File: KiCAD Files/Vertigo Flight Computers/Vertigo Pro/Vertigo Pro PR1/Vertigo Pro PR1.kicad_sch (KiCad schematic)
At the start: 152 parts, among them IC1 ICM-20602, IC2 DPS310XTSA1, J1 ST-LINK Conn, J2 USB_C_Receptacle_USB2.0, J3 FFC2A32-24-T, J4 Screw_Terminal, J5 Screw_Terminal, J6 Screw_Terminal, J7 Screw_Terminal, Q1 IRF530SPBF, Q2 MMBT3904-TP, Q3 MMBT3904-TP, Q4 IRF530SPBF, Q5 SI7149ADP-T1-GE3, Q6 MMBT3904-TP, Q7 MMBT3904-TP, Q8 IRF530SPBF, Q9 IRF530SPBF, SW1 SW_SPDT, U1 STM32F103C8Tx, U10 TPS79133DBVR, U11 TLV709, U12 TLV709, U13 TLV75528PDBV, U2 AP63203WU, U3 ESP32-S3-WROOM-1, U4 TLV75515PDBV, U5 LSM6DSO32, U7 TPS2121RUXR, U8 NEO-6M-GPS, U9 24AA32A-I_MS, Y1 16MHz

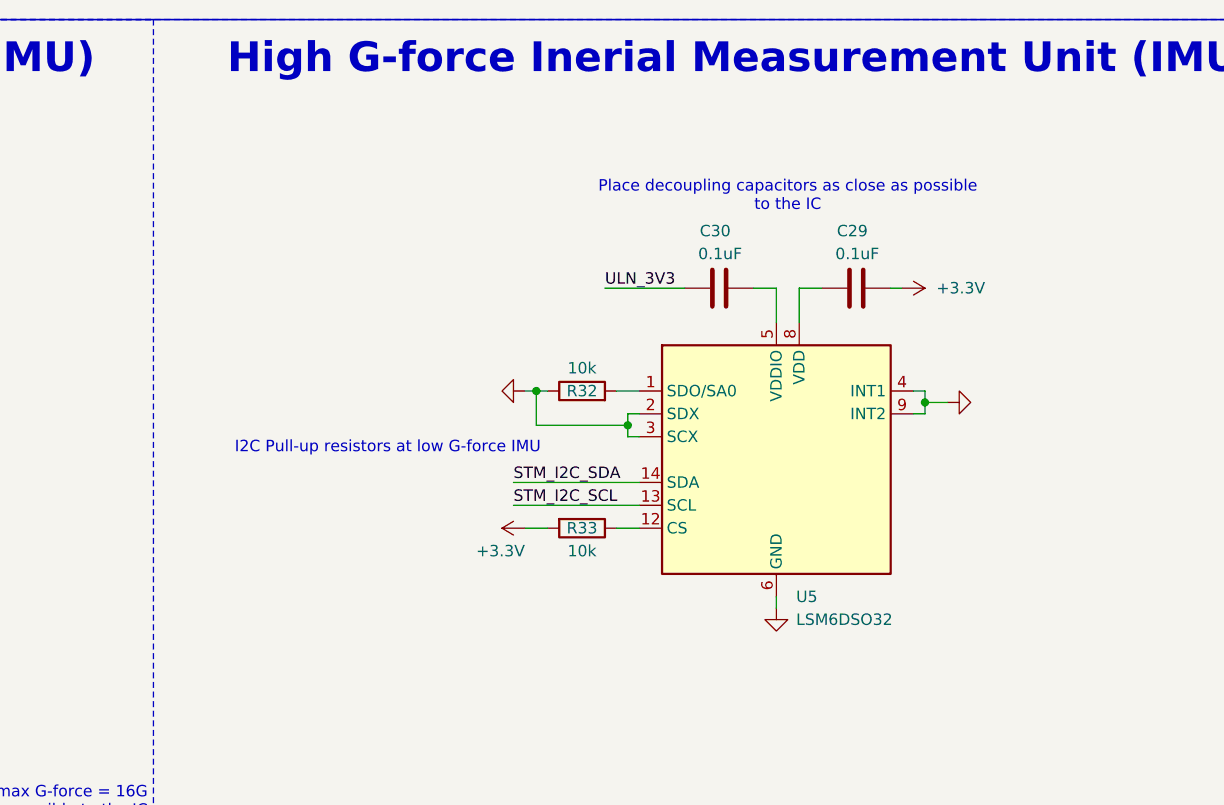
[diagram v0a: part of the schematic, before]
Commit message: Fix
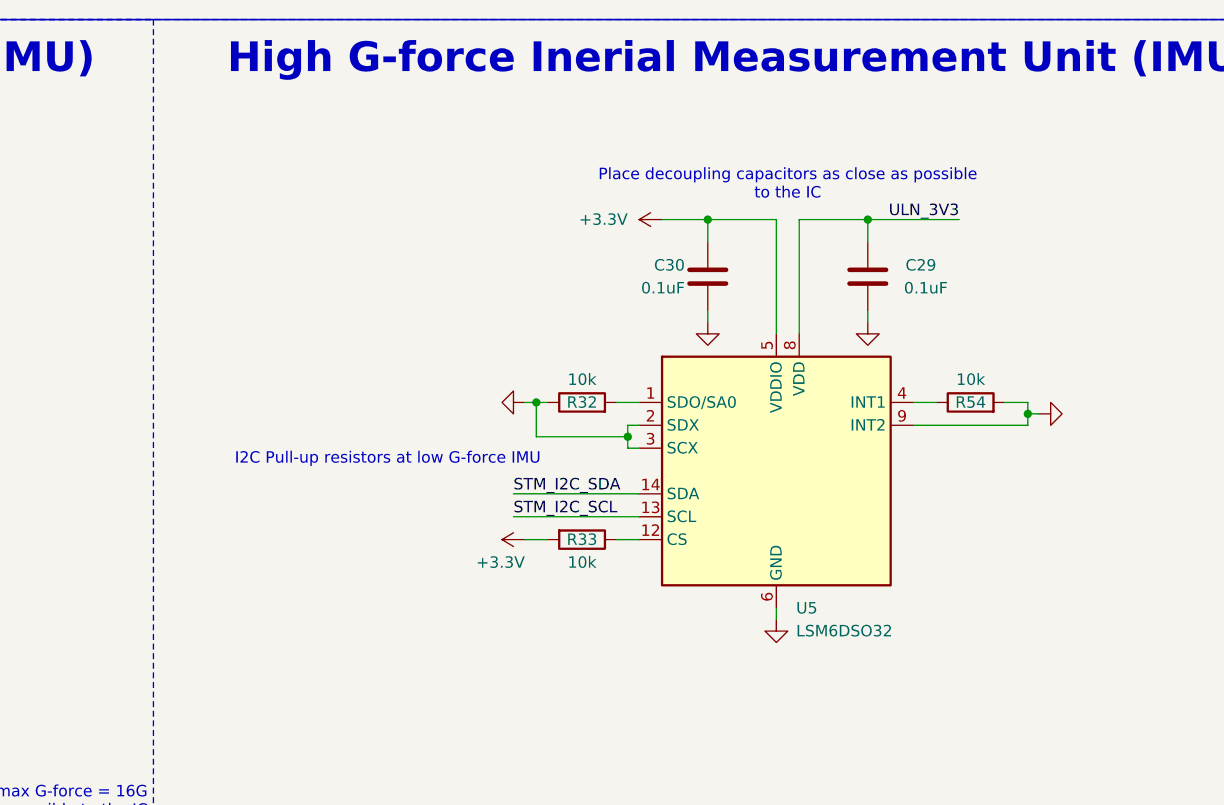
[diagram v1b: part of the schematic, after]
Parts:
- added R54: 10k, Resistor_SMD:R_1206_3216Metric, symbol Device:R
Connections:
- net +3.3V: now also C30.2, U5.5 (VDDIO); no longer C29.2
- net AGND: now also C29.1, C30.1, R54.2; no longer U5.4 (INT1)
- net ULN_3V3: now also C29.2, U5.8 (VDD); no longer C30.1
- new net: R54.1, U5.4 (INT1)
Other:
- moved on the sheet: C29, C30, R32, R33, U5
